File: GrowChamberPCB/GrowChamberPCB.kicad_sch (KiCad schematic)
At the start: 82 parts, among them J1 Screw_Terminal_01x02, J10 Screw_Terminal_01x03, J27 Conn_01x26_Pin, J3 TYPE-C-31-M-12, J7 Screw_Terminal_01x05, Q1 IRLML6244, Q2 IRLML6244, Q3 IRLML6244, Q4 IRLML6244, Q5 IRLML6244, Q6 IRLML6244, Q7 IRLR8721, Q9 IRLML6244, SW3 BootMode_Switch, SW5 ResetButton_Internal, U1 ESP32-S3-WROOM-1U, U2 MCP1826S, U3 USBLC6-2SC6, U4 TC4428EOA, U5 W25Q128JVS, U6 CR2013-MI2120

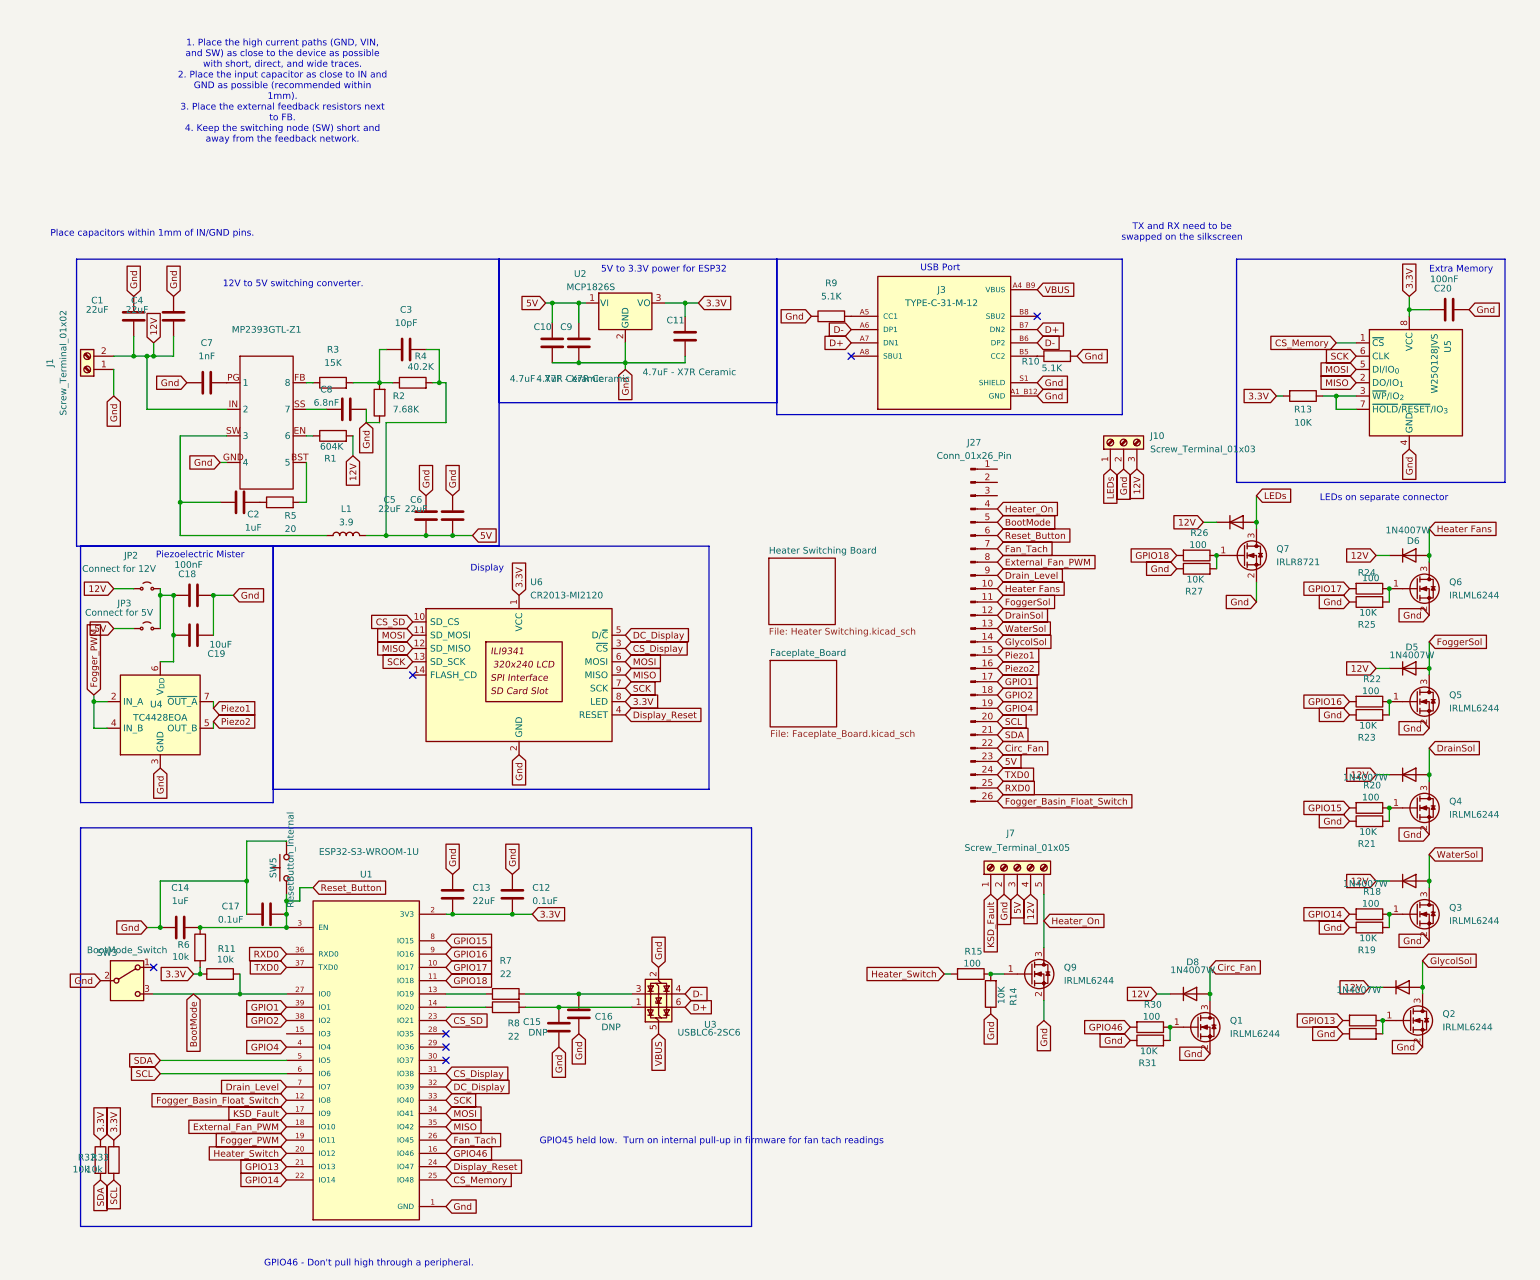
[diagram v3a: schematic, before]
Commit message: working on stuff
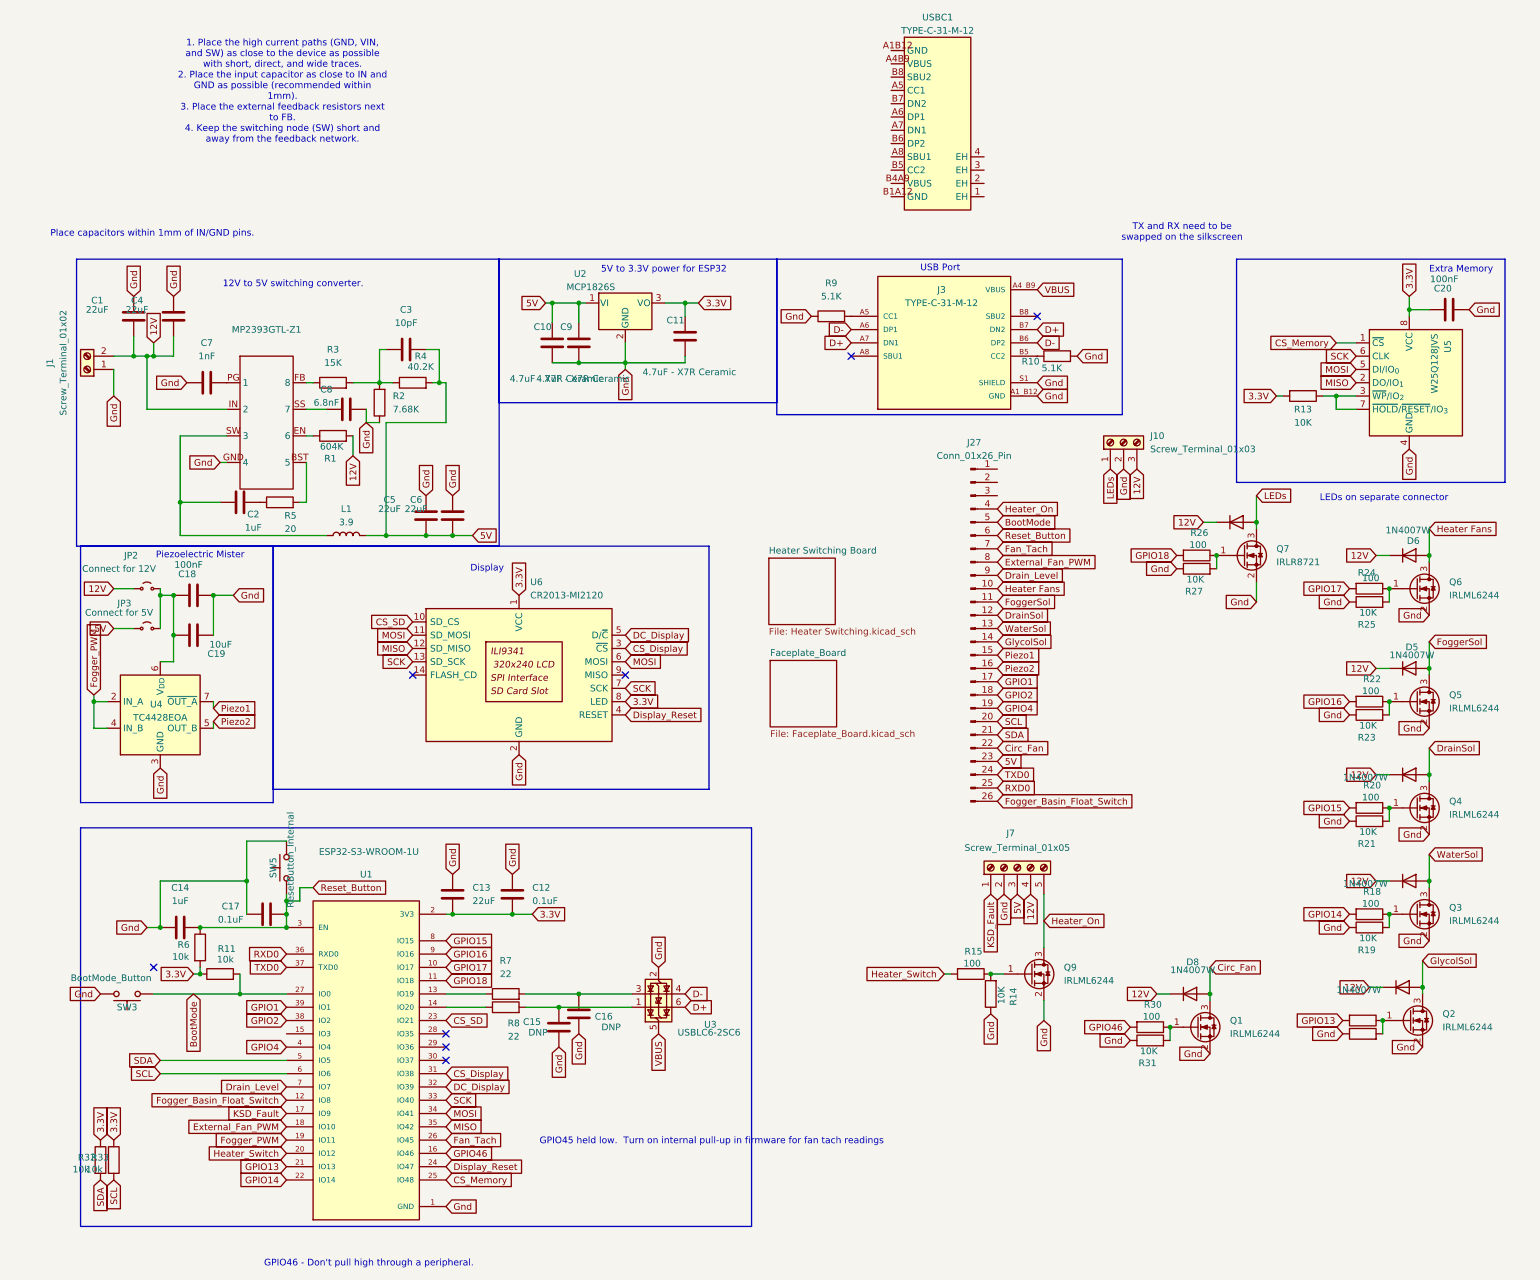
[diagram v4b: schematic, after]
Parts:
- removed SW3: BootMode_Switch, symbol Switch:SW_SPDT
- added SW3: BootMode_Button, Button_Switch_SMD:SW_Push_1P1T_XKB_TS-1187A, symbol Switch:SW_Push
- added USBC1: TYPE-C-31-M-12, easyeda2kicad:USB-C_SMD-TYPE-C-31-M-12_1, symbol easyeda2kicad:TYPE-C-31-M-12
- U1: footprint (none) -> PCM_Espressif:ESP32-S3-WROOM-1U; MFG Part Number (none) -> ESP32-S3-WROOM-1U-N8R8; Manufacturer (none) -> Espressif Systems; Package (none) -> SMD,19.2x18mm; Type (SMD/thru-hole, etc.) (none) -> SMD
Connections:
- net BootMode: now also SW3.1
- net GND: now also SW3.2; no longer U1.41_1 (GND), U1.41_2 (GND), U1.41_3 (GND), U1.41_4 (GND), U1.41_5 (GND), U1.41_6 (GND), U1.41_7 (GND), U1.41_8 (GND), U1.41_9 (GND)
- net MISO: no longer U6.9 (MISO)
- no-connect marks 7 -> 8
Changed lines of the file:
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@@
 	)
 	(no_connect
+		(at 116.84 91.44)
+	)
+	(no_connect
 		(at 195.58 22.86)
 	)
@@
 	(global_label "Gnd"
 		(shape input)
-		(at 16.51 149.86 180)
+		(at 16.51 152.4 180)
 		(fields_autoplaced yes)
 		(effects
@@
 		)
 		(property "Intersheetrefs" "${INTERSHEET_REFS}"
-			(at 9.9568 149.86 0)
+			(at 9.9568 152.4 0)
 			(effects
 				(font
@@
 		)
 	)
-	(global_label "MISO"
-		(shape input)
-		(at 116.84 91.44 0)
-		(fields_autoplaced yes)
-		(effects
-			(font
-				(size 1.27 1.27)
-			)
-			(justify left)
-		)
-		(property "Intersheetrefs" "${INTERSHEET_REFS}"
-			(at 124.4214 91.44 0)
-			(effects
-				(font
-					(size 1.27 1.27)
-				)
-				(justify left)
-				(hide yes)
-			)
-		)
-	)
 	(global_label "SCK"
 		(shape input)
@@
 	)
 	(symbol
+		(lib_id "Switch:SW_Push")
+		(at 21.59 152.4 180)
+		(unit 1)
+		(exclude_from_sim no)
+		(in_bom yes)
+		(on_board yes)
+		(dnp no)
+		(property "Reference" "SW3"
+			(at 21.59 154.94 0)
+			(effects
+				(font
+					(size 1.27 1.27)
+				)
+			)
+		)
+		(property "Value" "BootMode_Button"
+			(at 18.542 149.352 0)
+			(effects
+				(font
+					(size 1.27 1.27)
+				)
+			)
+		)
+		(property "Footprint" "Button_Switch_SMD:SW_Push_1P1T_XKB_TS-1187A"
+			(at 21.59 157.48 0)
+			(effects
+				(font
+					(size 1.27 1.27)
+				)
+				(hide yes)
+			)
+		)
+		(property "Datasheet" "https://jlc-prod-smt.oss-eu-central-1.aliyuncs.com/smtDataManualFile/8550724022091735040-C318884.pdf?response-content-disposition=attachment%3B%20filename%3DC318884.pdf%3B%20filename%2A%3DUTF-8%27%27C318884.pdf&x-oss-date=20260623T203203Z&x-oss-expires=1800&x-oss-security-token=CAISgAN1q6Ft5B2yfSjIr5vsPfTmrKdi%2Ba%2FYOlD8nU0nar5i3fTulTz2IHhMdHJsAOodtv0%2FmmhT6PkclqRLcbhpcmfjV%2BZHzLB8qepJv1ZG4J7b16cNrbH4M4H6aXeirtuwDsz9SNTCALjPD3nPii50x5bjaDymRCbLGJaViJlhHLN1Ow6jdmhpCctxLAlvo9NgFxm3D%2Fu2NQPwiWf9FVdhvhEG6Vly8qOi2MaRmFy8yFTx0b0SvJ%2BjYMrmPctoN9JnSdC5mfdzau3a1TJ84gRD0a5wkaVA1zbDs5bfISEIuUzebreLqY03dV4mOvdqIcMe8qigz88fk%2FfIioH6xyxKOexoSCnFTOiiupCcQLPyao9jLu6iayqViY7QaIOTqQohZmkAMwVOasAsI3Ngh4zF97Qt0cVNkXO9gWfLI8DtuMleWpohUVpD7tHD0eS19jklBdzSlusJRAJJUVBflCeKEaRNSAd3WGhEfM2%2BBt4QT30w5N2u00S8OSMIzGHxnqKWD5sagAGwGdg7eBRMe%2BjpmZKoMN29EbI%2BqeGWDU%2BDN00Al2NVRqyAwYTC2%2BRN3r3KydJAsor2R%2BId%2Fl0%2FMQM8NLpR3Tl%2FttaRfEoqhy9ZHOrBuuyJcP8ULoQ3qLZ6xiB%2FQQRtxnhSFSTuxrRbCzjPg0RpjFkz%2FPFgFCM03kfF1QwKI%2FFgsCAA&x-oss-signature-version=OSS4-HMAC-SHA256&x-oss-credential=STS.NXYvNRAxCNm38vMyMrf1N21Ew%2F20260623%2Feu-central-1%2Foss%2Faliyun_v4_request&x-oss-signature=e43aa02dab2f35991183760960ab48201f603011864f04475b1513b165997cdf"
+			(at 21.59 157.48 0)
+			(effects
+				(font
+					(size 1.27 1.27)
+				)
+				(hide yes)
+			)
+		)
+		(property "Description" "Push button switch, generic, two pins"
+			(at 21.59 152.4 0)
+			(effects
+				(font
+					(size 1.27 1.27)
+				)
+				(hide yes)
+			)
+		)
+		(property "MFG Part Number" "TS-1187A-B-A-B "
+			(at 21.59 152.4 0)
+			(effects
+				(font
+					(size 1.27 1.27)
+				)
+				(hide yes)
+			)
+		)
+		(property "Type (SMD/thru-hole, etc.)" "SMD"
+			(at 21.59 152.4 0)
+			(effects
+				(font
+					(size 1.27 1.27)
+				)
+				(hide yes)
+			)
+		)
+		(property "Manufacturer" "XKB Connection"
+			(at 21.59 152.4 0)
+			(effects
+				(font
+					(size 1.27 1.27)
+				)
+				(hide yes)
+			)
+		)
+		(property "Package" "SMD-4P,5.1x5.1mm "
+			(at 21.59 152.4 0)
+			(effects
+				(font
+					(size 1.27 1.27)
+				)
+				(hide yes)
+			)
+		)
+		(pin "2"
+		)
+		(pin "1"
+		)
+		(instances
+			(project "GrowChamberPCB"
+				(path "/39371779-5336-4073-adec-fb32caf6a86f"
+					(reference "SW3")
+					(unit 1)
+				)
+			)
+		)
+	)
+	(symbol
 		(lib_id "Device:R")
 		(at 69.85 39.37 180)
@@
 			)
 		)
-		(property "Footprint" ""
+		(property "Footprint" "PCM_Espressif:ESP32-S3-WROOM-1U"
 			(at 67.31 165.1 0)
 			(effects
@@
 			)
 		)
-		(property "Description" ""
+		(property "Description" "microcontroller"
 			(at 67.31 165.1 0)
 			(effects
@@
 			)
 		)
-		(property "MFG Part Number" ""
+		(property "MFG Part Number" "ESP32-S3-WROOM-1U-N8R8 "
 			(at 67.31 165.1 0)
 			(effects
@@
 			)
 		)
-		(property "Type (SMD/thru-hole, etc.)" ""
+		(property "Type (SMD/thru-hole, etc.)" "SMD"
 			(at 67.31 165.1 0)
 			(effects
@@
 			)
 		)
-		(property "Manufacturer" ""
+		(property "Manufacturer" "Espressif Systems"
 			(at 67.31 165.1 0)
 			(effects
@@
 			)
 		)
-		(property "Package" ""
+		(property "Package" "SMD,19.2x18mm"
 			(at 67.31 165.1 0)
 			(effects
@@
 		(pin "1"
 		)
-		(pin "41_3"
-		)
-		(pin "41_2"
-		)
-		(pin "41_6"
-		)
 		(pin "34"
 		)
 		(pin "25"
 		)
-		(pin "41_4"
-		)
 		(pin "24"
 		)
-		(pin "41_8"
-		)
 		(pin "33"
 		)
@@
 		(pin "40"
 		)
-		(pin "41_5"
-		)
 		(pin "32"
 		)
-		(pin "41_7"
-		)
 		(pin "35"
 		)
-		(pin "41_9"
-		)
 		(pin "26"
 		)
-		(pin "41_1"
-		)
 		(instances
 			(project "GrowChamberPCB"
@@
 	)
 	(symbol
+		(lib_id "easyeda2kicad:TYPE-C-31-M-12")
+		(at 173.99 -13.97 0)
+		(unit 1)
+		(exclude_from_sim no)
+		(in_bom yes)
+		(on_board yes)
+		(dnp no)
+		(fields_autoplaced yes)
+		(property "Reference" "USBC1"
+			(at 176.53 -34.29 0)
+			(effects
+				(font
+					(size 1.27 1.27)
+				)
+			)
+		)
+		(property "Value" "TYPE-C-31-M-12"
+			(at 176.53 -31.75 0)
+			(effects
+				(font
+					(size 1.27 1.27)
+				)
+			)
+		)
+		(property "Footprint" "easyeda2kicad:USB-C_SMD-TYPE-C-31-M-12_1"
+			(at 173.99 7.62 0)
+			(effects
+				(font
+					(size 1.27 1.27)
+				)
+				(hide yes)
+			)
+		)
+		(property "Datasheet" "https://lcsc.com/product-detail/USB-Type-C_Korean-Hroparts-Elec-TYPE-C-31-M-12_C165948.html"
+			(at 173.99 10.16 0)
+			(effects
+				(font
+					(size 1.27 1.27)
+				)
+				(hide yes)
+			)
+		)
+		(property "Description" ""
+			(at 173.99 -13.97 0)
+			(effects
+				(font
+					(size 1.27 1.27)
+				)
+				(hide yes)
+			)
+		)
+		(property "Manufacturer" "韩国韩荣"
+			(at 173.99 12.7 0)
+			(effects
+				(font
+					(size 1.27 1.27)
+				)
+				(hide yes)
+			)
+		)
+		(property "MPN" "TYPE-C-31-M-12"
+			(at 173.99 15.24 0)
+			(effects
+				(font
+					(size 1.27 1.27)
+				)
+				(hide yes)
+			)
+		)
+		(property "LCSC Part" "C165948"
+			(at 173.99 17.78 0)
+			(effects
+				(font
+					(size 1.27 1.27)
+				)
+				(hide yes)
+			)
+		)
+		(pin "B4A9"
+		)
+		(pin "1"
+		)
+		(pin "A8"
+		)
+		(pin "2"
+		)
+		(pin "B1A12"
+		)
+		(pin "B5"
+		)
+		(pin "4"
+		)
+		(pin "B6"
+		)
+		(pin "A4B9"
+		)
+		(pin "A1B12"
+		)
+		(pin "B8"
+		)
+		(pin "A6"
+		)
+		(pin "B7"
+		)
+		(pin "A5"
+		)
+		(pin "3"
+		)
+		(pin "A7"
+		)
+		(instances
+			(project "GrowChamberPCB"
+				(path "/39371779-5336-4073-adec-fb32caf6a86f"
+					(reference "USBC1")
+					(unit 1)
+				)
+			)
+		)
+	)
+	(symbol
 		(lib_id "Device:C")
 		(at 48.26 137.16 90)
@@
 					(unit 1)
 				)
-			)
-		)
-	)
-	(symbol
-		(lib_id "Switch:SW_SPDT")
-		(at 21.59 149.86 0)
-		(unit 1)
-		(exclude_from_sim no)
-		(in_bom yes)
-		(on_board yes)
-		(dnp no)
-		(property "Reference" "SW3"
-			(at 17.78 144.526 0)
-			(effects
-				(font
-					(size 1.27 1.27)
-				)
-			)
-		)
-		(property "Value" "BootMode_Switch"
-			(at 21.59 144.018 0)
-			(effects
-				(font
-					(size 1.27 1.27)
-				)
-			)
-		)
-		(property "Footprint" ""
-			(at 21.59 149.86 0)
-			(effects
-				(font
-					(size 1.27 1.27)
-				)
-				(hide yes)
-			)
-		)
-		(property "Datasheet" "~"
-			(at 21.59 157.48 0)
-			(effects
-				(font
-					(size 1.27 1.27)
-				)
-				(hide yes)
-			)
-		)
-		(property "Description" "Switch, single pole double throw"
-			(at 21.59 149.86 0)
-			(effects
-				(font
-					(size 1.27 1.27)
-				)
-				(hide yes)
-			)
-		)
-		(property "MFG Part Number" ""
-			(at 21.59 149.86 0)
-			(effects
-				(font
-					(size 1.27 1.27)
-				)
-				(hide yes)
-			)
-		)
-		(pin "1"
-		)
-		(pin "3"
-		)
-		(pin "2"
-		)
-		(instances
-			(project "GrowChamberPCB"
-				(path "/39371779-5336-4073-adec-fb32caf6a86f"
-					(reference "SW3")
-					(unit 1)
-				)
